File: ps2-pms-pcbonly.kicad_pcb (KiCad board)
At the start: 2 copper layers, 93.9 x 47 mm, 283 parts, among them U1 ADP151, U2 SC174, U3 TPS61253, U4 BQ24076, U5 CSD22202W15

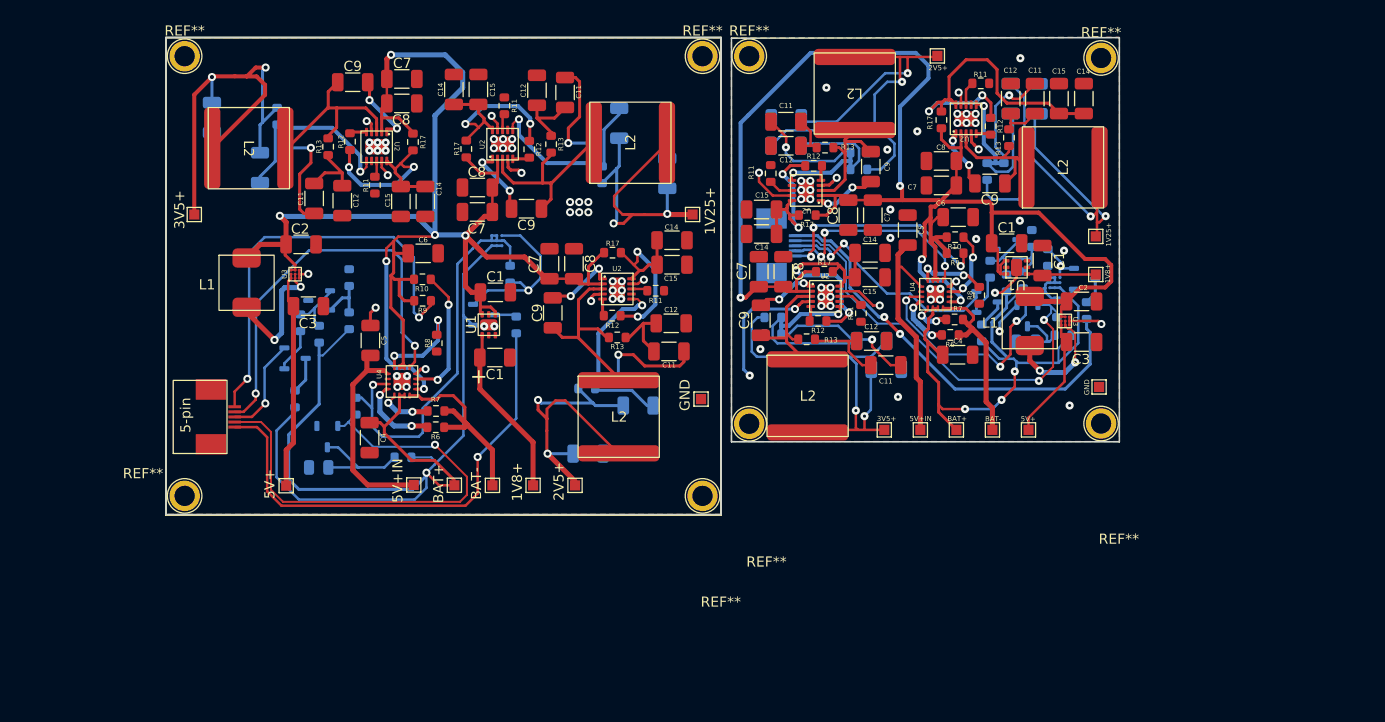
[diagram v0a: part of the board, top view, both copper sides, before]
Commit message: build(final-push): final push
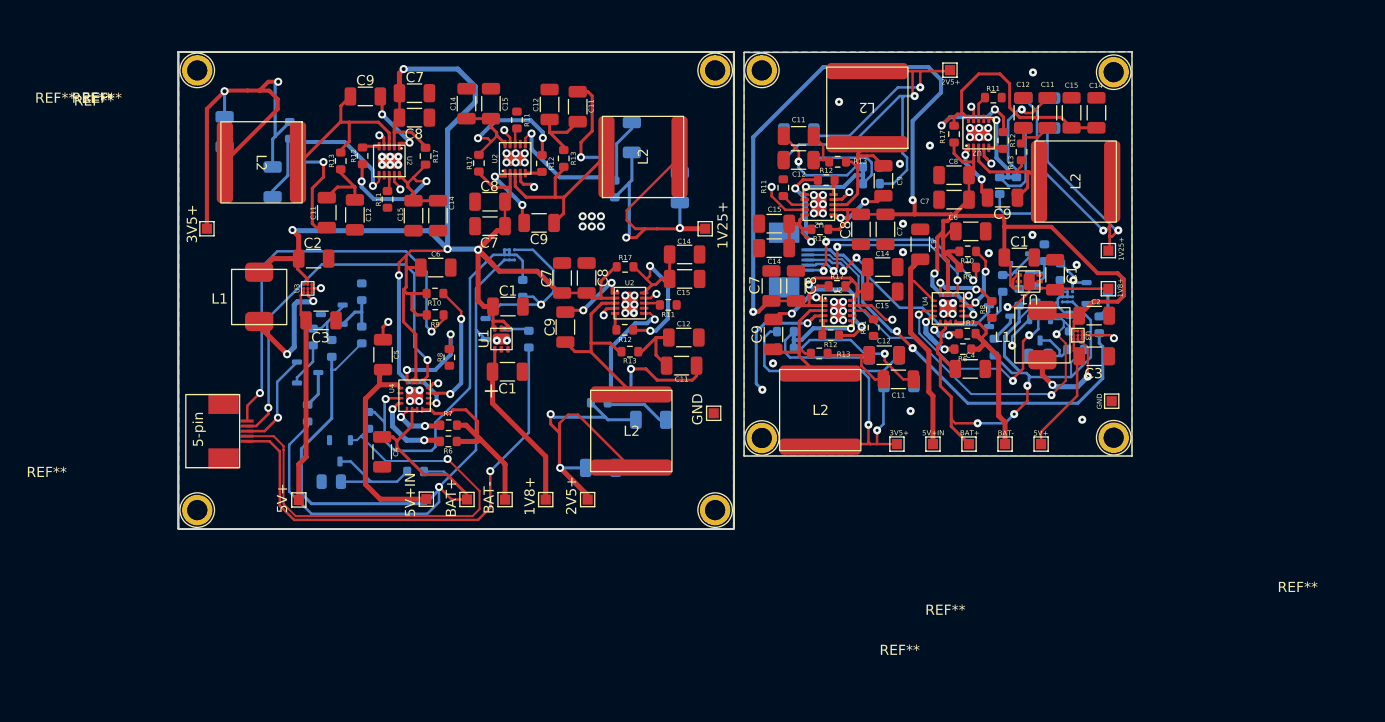
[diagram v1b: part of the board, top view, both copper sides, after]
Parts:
- moved R12 1.87 mm to (58.0, 41.4)
- moved U1 1.87 mm to (97.9, 36.6)
- moved U2 1.87 mm to (79.0, 39.5)
- moved 1V25+ 1.87 mm to (66.0, 31.4)
- moved C10 1.87 mm to (97.3, 20.0)
- moved C11 1.87 mm to (99.7, 20.0)
- moved C12 1.87 mm to (97.3, 20.0)
- moved C14 1.87 mm to (104.5, 20.0)
- moved C15 1.87 mm to (102.0, 20.0)
- moved C7 1.87 mm to (90.5, 28.5)
- moved C8 1.87 mm to (90.5, 26.1)
- moved C9 1.87 mm to (83.5, 26.7)
- moved C9 1.87 mm to (95.2, 28.3)
- moved L2 1.87 mm to (81.9, 19.5)
- moved R11 1.87 mm to (94.3, 18.5)
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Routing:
- net 2V5+: track 131.4 -> 133.1 mm
